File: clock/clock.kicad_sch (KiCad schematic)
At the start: 4 parts

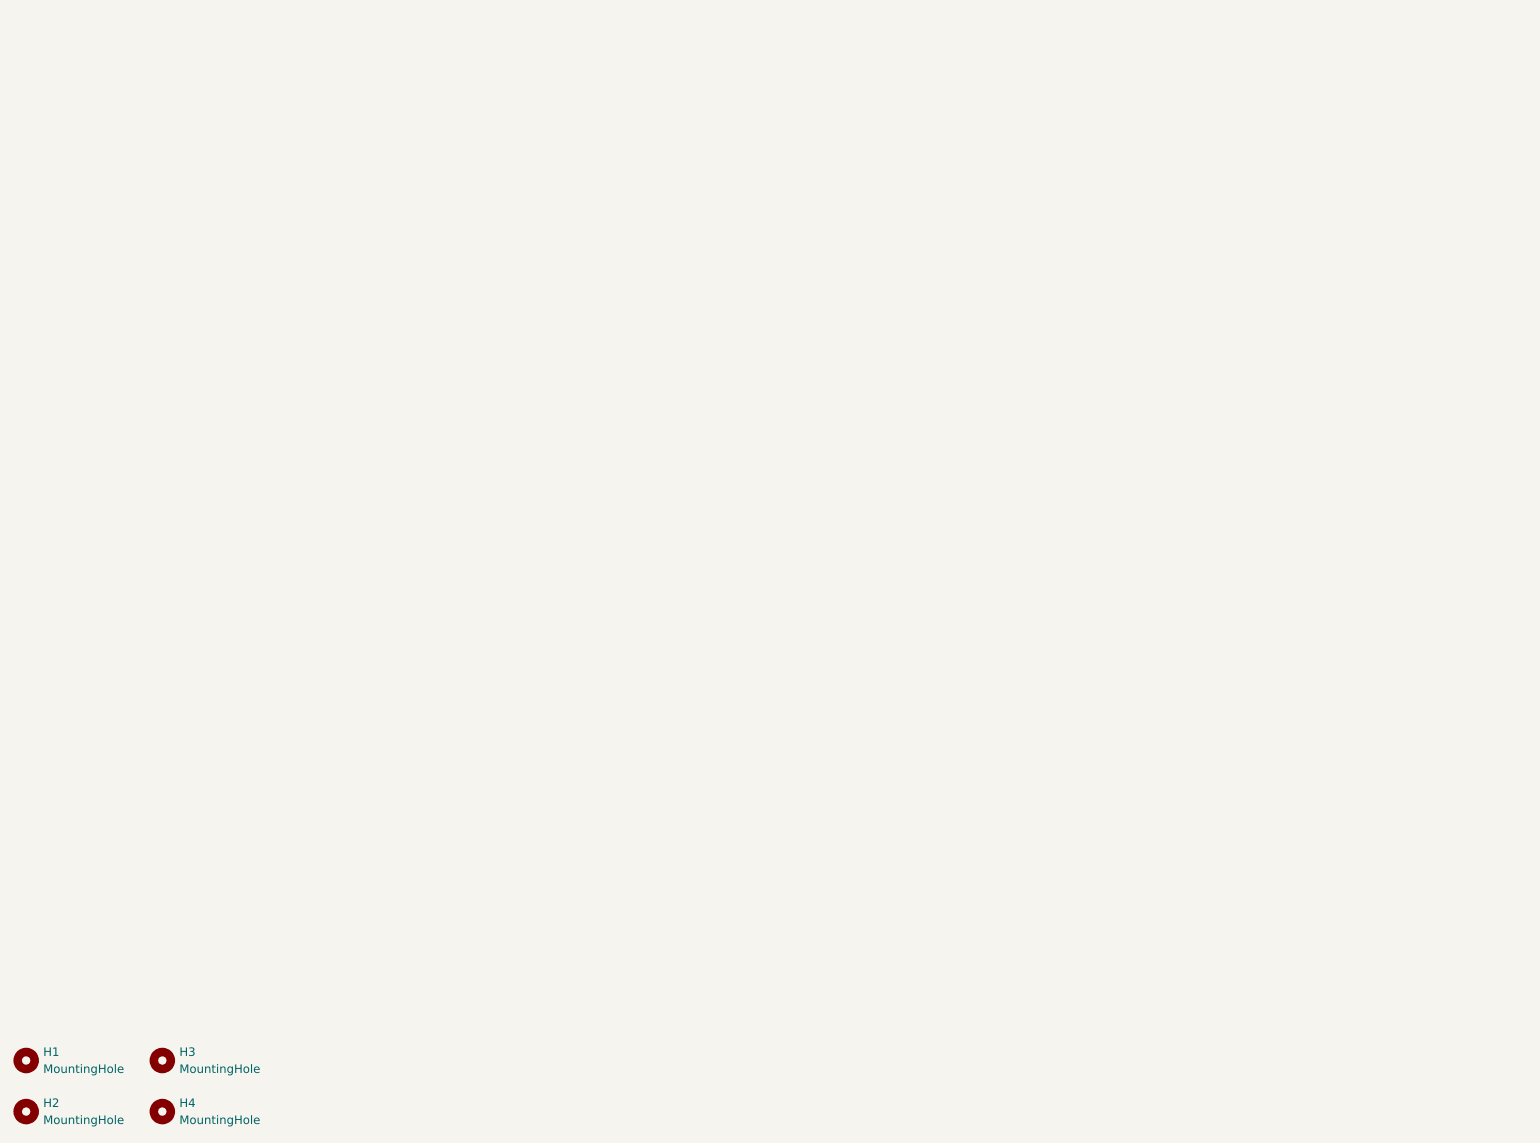
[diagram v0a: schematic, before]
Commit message: Blinky Led
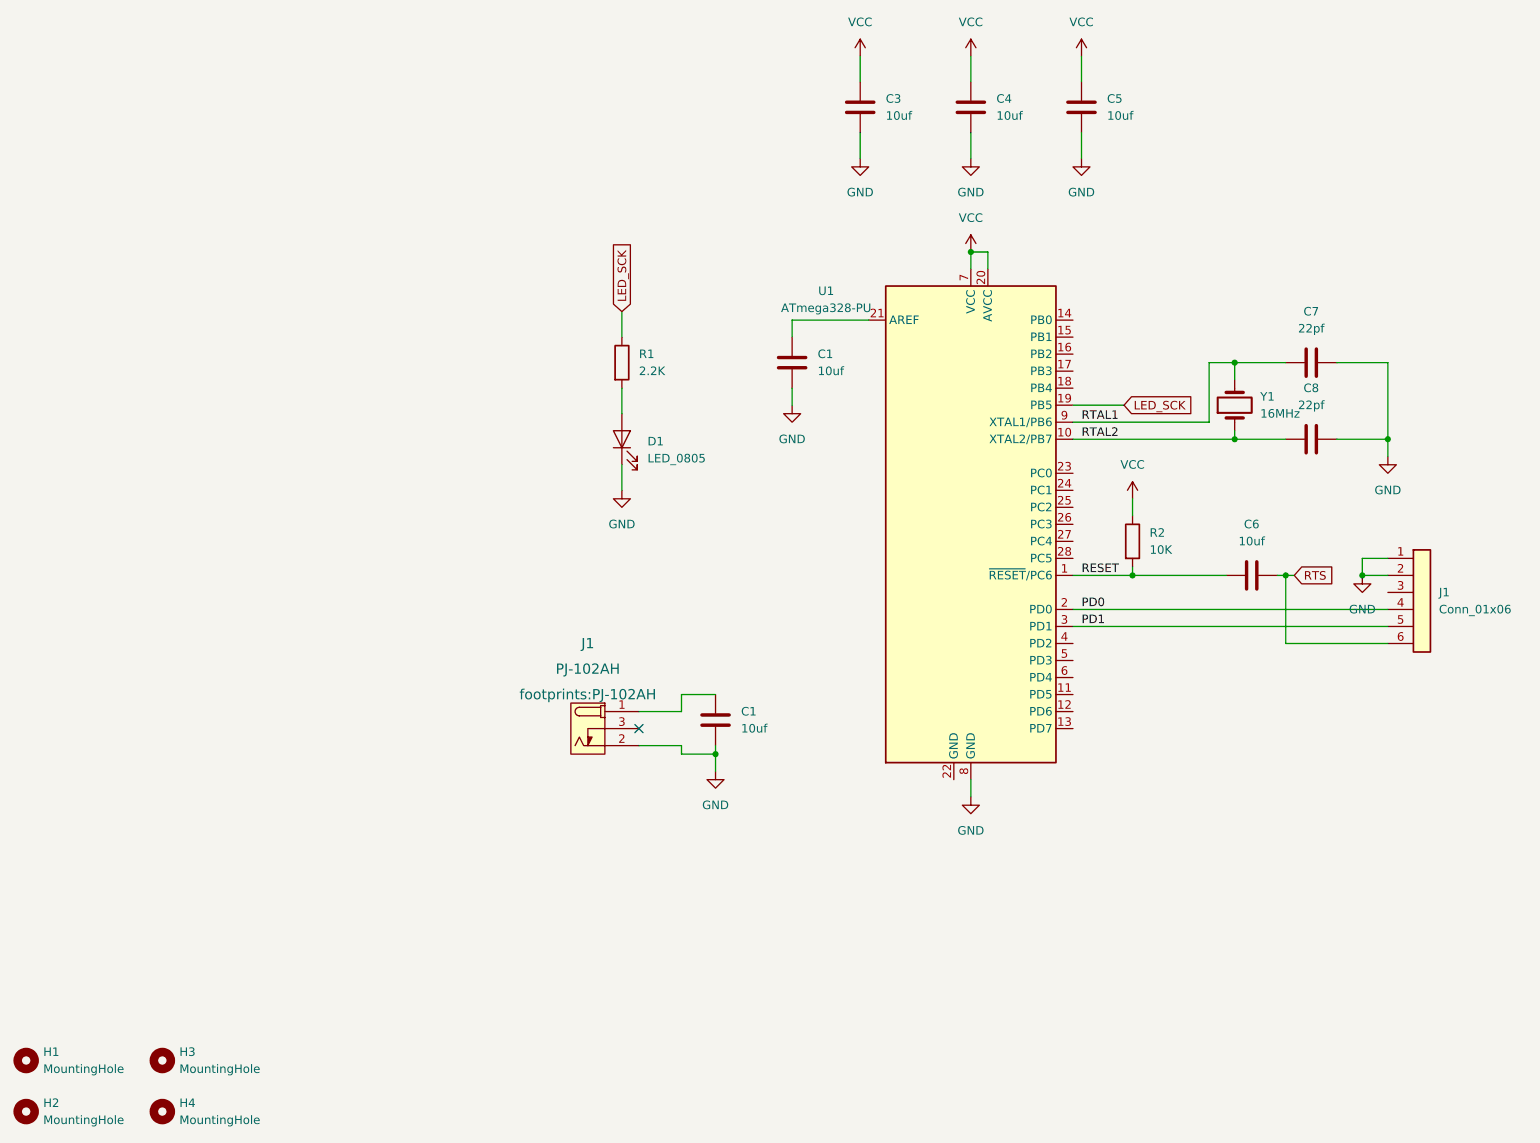
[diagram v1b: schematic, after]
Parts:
- added C1 (x2), C3, C4, C5, C6: 10uf, footprints:C_0805_2012Metric, symbol HPS:C_0805_10uf
- added C7, C8: 22pf, footprints:C_0805_2012Metric, symbol HPS:C_0805_22pf
- added D1: LED_0805, footprints:LED_0805_2012Metric, symbol HPS:LED_0805
- added J1: Conn_01x06, footprints:PinHeader_1x06_P2.54mm_Vertical, symbol HPS:Conn_01x06
- added J1: PJ-102AH, footprints:PJ-102AH, symbol HPS:PJ-102AH
- added R1: 2.2K, footprints:R_0805_2012Metric, symbol HPS:R_0805_2.2K
- added R2: 10K, footprints:R_0805_2012Metric, symbol HPS:R_0805_10K
- added U1: ATmega328-PU, footprints:DIP-28_W7.62mm, symbol HPS:ATmega328-PU
- added Y1: 16MHz, footprints:Crystal_SMD_HC49-SD, symbol HPS:Crystal_16MHz
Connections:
- new net: D1.2 (A), R1.2
- new net: C1.1, J1.1 (POLE)
- new net: C1.1, U1.21 (AREF)
- new net GND: C1.2, C1.2, C3.2, C4.2, C5.2, C7.1, C8.1, D1.1 (K), J1.1 (Pin_1), J1.2 (OUT), J1.2 (Pin_2), U1.8 (GND)
- new net LED_SCK: R1.1, U1.19 (PB5)
- new net PD0: J1.4 (Pin_4), U1.2 (PD0)
- new net PD1: J1.5 (Pin_5), U1.3 (PD1)
- new net RESET: C6.2, R2.2, U1.1 (~{RESET}/PC6)
- new net RTAL1: C7.2, U1.9 (XTAL1/PB6), Y1.2
- new net RTAL2: C8.2, U1.10 (XTAL2/PB7), Y1.1
- new net RTS: C6.1, J1.6 (Pin_6)
- new net VCC: C3.1, C4.1, C5.1, R2.1, U1.20 (AVCC), U1.7 (VCC)
- no-connect marks 0 -> 1
